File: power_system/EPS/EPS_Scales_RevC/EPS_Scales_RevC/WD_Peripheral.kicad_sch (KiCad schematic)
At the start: 35 parts, among them J16 Conn_01x04, U13 TLV1704

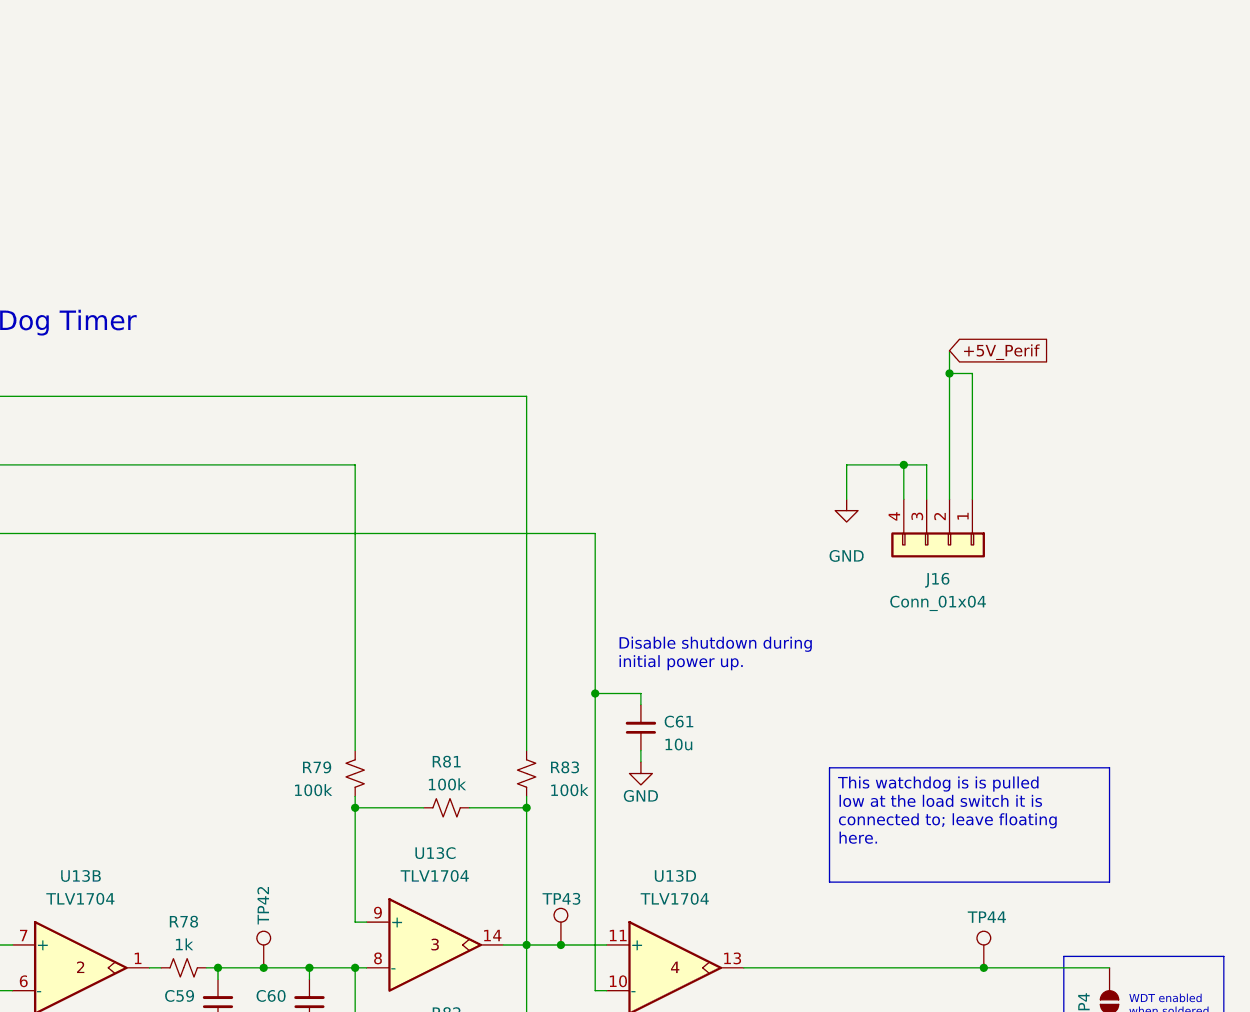
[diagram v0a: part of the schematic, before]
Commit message: Revert "Luca branch v2"
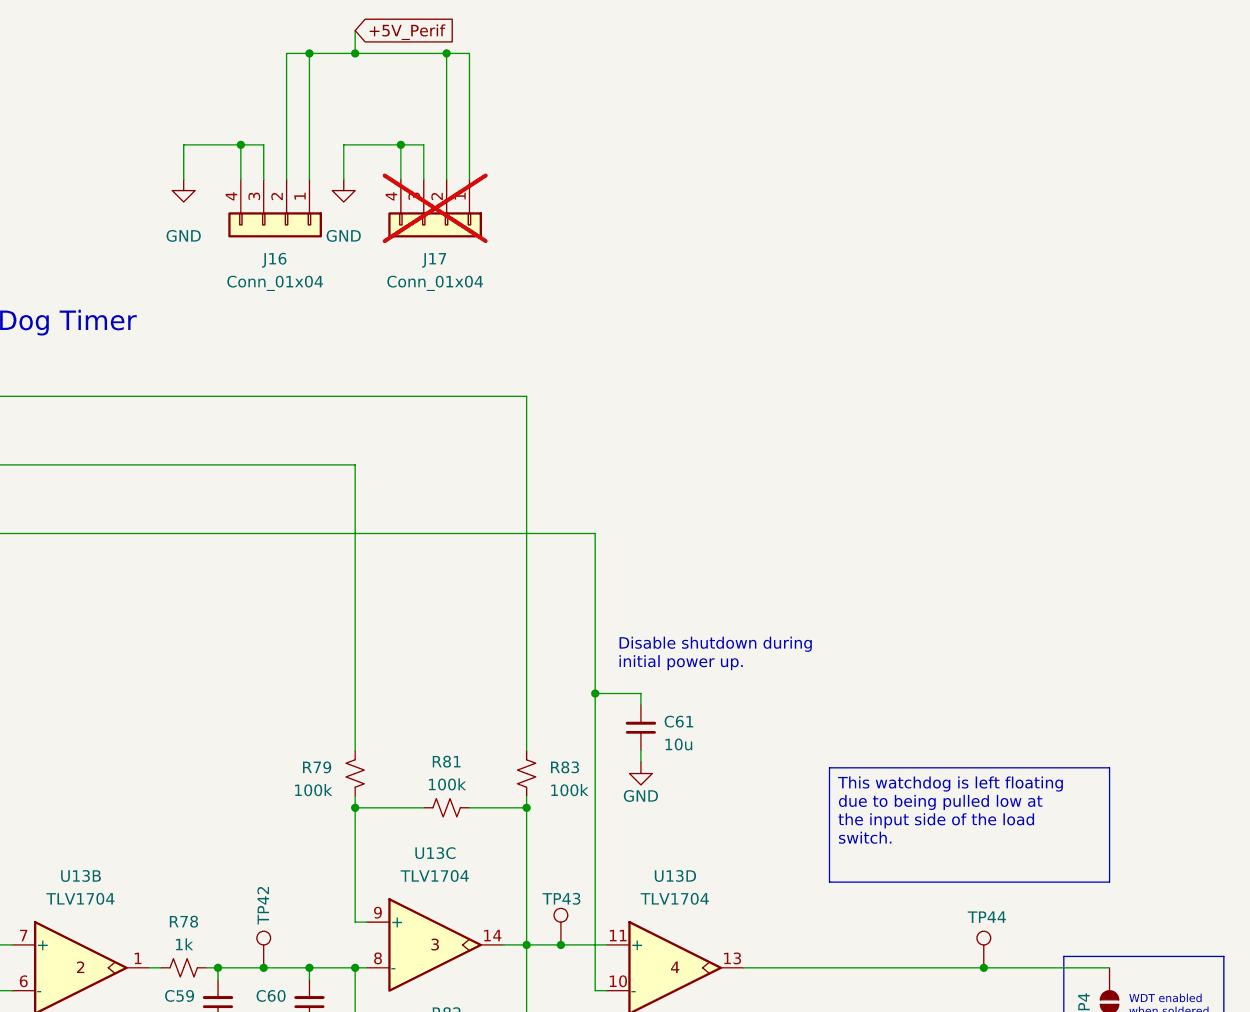
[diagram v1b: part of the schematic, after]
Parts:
- added J17: Conn_01x04, Connector_PinSocket_2.54mm:PinSocket_1x04_P2.54mm_Vertical, symbol Connector_Generic:Conn_01x04
- D7, D9: footprint RevC Footprints:SODFL2512X100N -> Diode_SMD:D_SOD-323
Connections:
- net +5V_Perif: now also J17.1 (Pin_1), J17.2 (Pin_2)
- net GND: now also J17.3 (Pin_3), J17.4 (Pin_4)
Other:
- moved on the sheet: J16
